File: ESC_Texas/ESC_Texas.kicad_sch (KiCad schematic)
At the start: 71 parts, among them IC1 nRF52840-QFAA-F-R7, IC11 LM3480IM3-3.3_NOPB, IC12 LM3480IM3-3.3_NOPB, J11 Battery+, J12 Conn_01x02, J14 USB_B_Micro, J2 RJ45, J3 Motor, J4 Battery+, P0.10 TestPoint, P0.11 TestPoint, P0.12 TestPoint, P0.18 TestPoint, P0.7 TestPoint, P0.9 TestPoint, P1.0 TestPoint, P1.9 TestPoint, U1 MCP2515-xSO, U2 TJA1051T, X1 CM7V-T1A-32.768kHz, X2 32MHz, X3 C115962

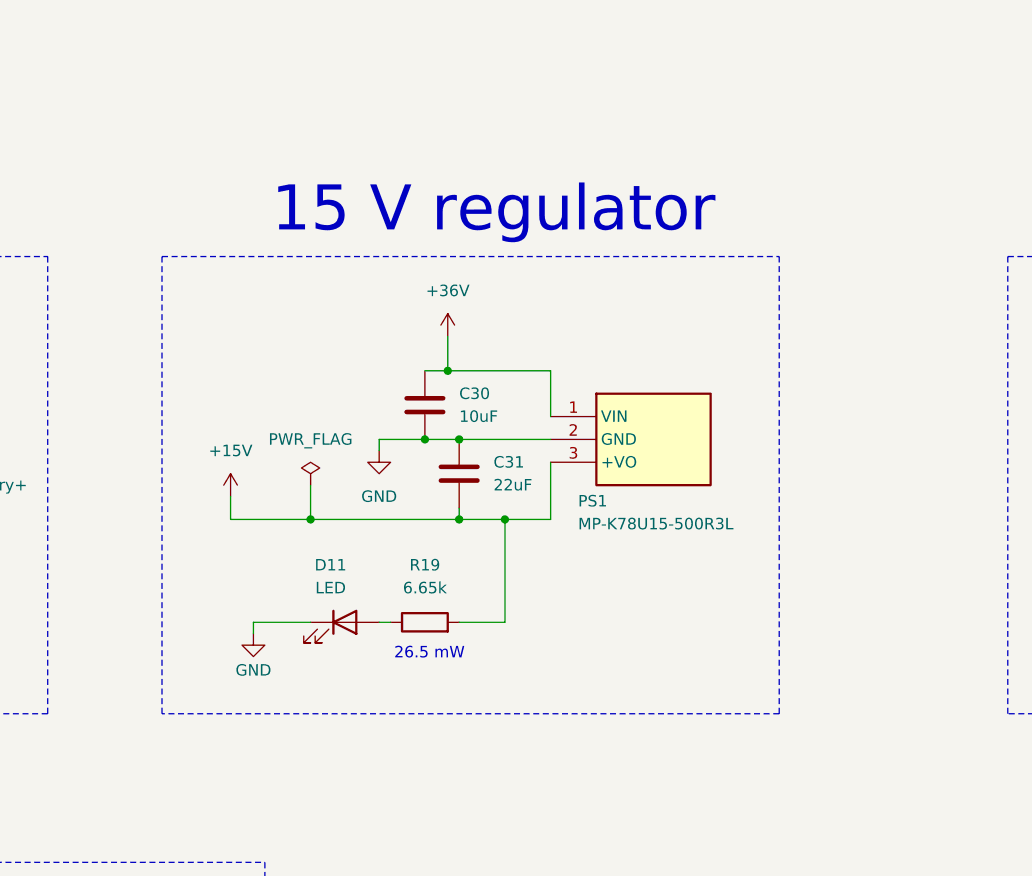
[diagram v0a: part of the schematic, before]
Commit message: Expanded heat thing
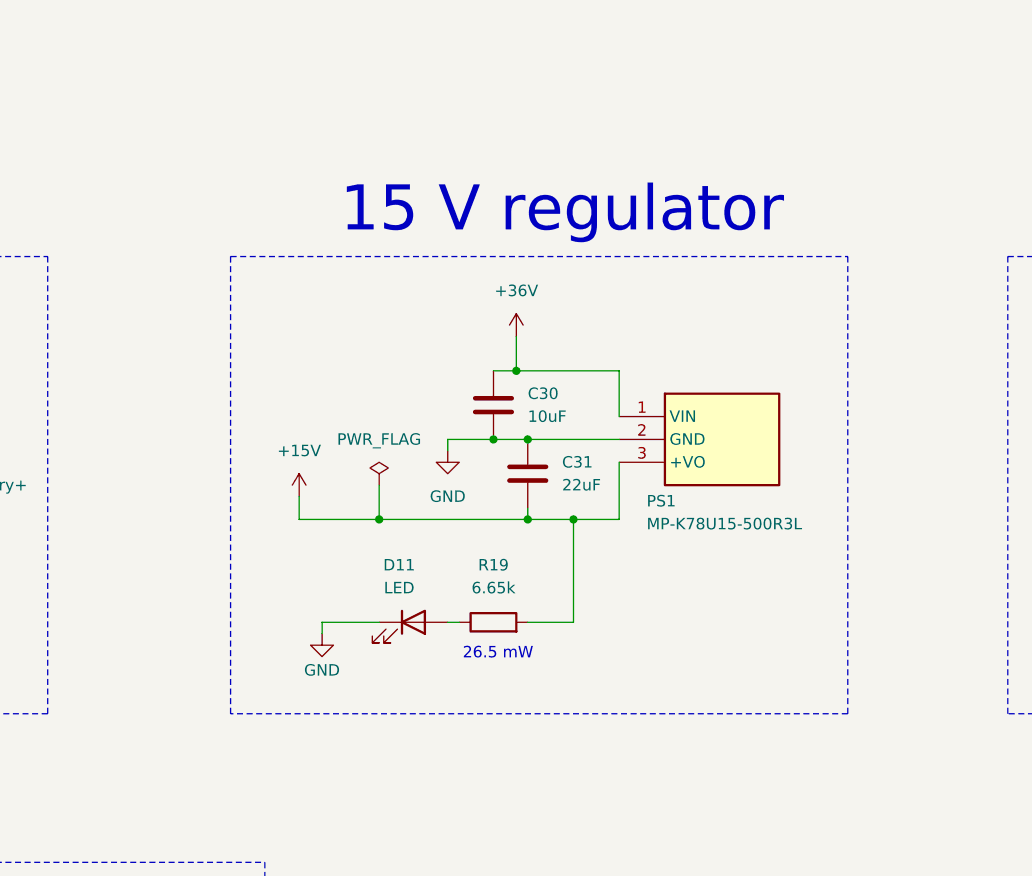
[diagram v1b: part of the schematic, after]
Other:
- moved on the sheet: C30, C31, D11, PS1, R19
